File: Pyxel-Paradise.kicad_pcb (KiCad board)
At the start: 2 copper layers, 61 x 63.5 mm, 33 parts, among them J1 Joystick-North, J10 Action-Up, J11 Action-Right, J12 Action-Down, J13 Action-Left, J14 Meta-Button-1, J15 Meta-Button-2, J16 Meta-Button-3, J17 Meta-Button-4, J2 Joystick-NorthEast, J3 Joystick-East, J4 Joystick-SouthEast, J5 Joystick-South, J6 Joystick-SouthWest, J7 Joystick-West, J8 Joystick-NorthWest, J9 Raspberry_Pi_2_3

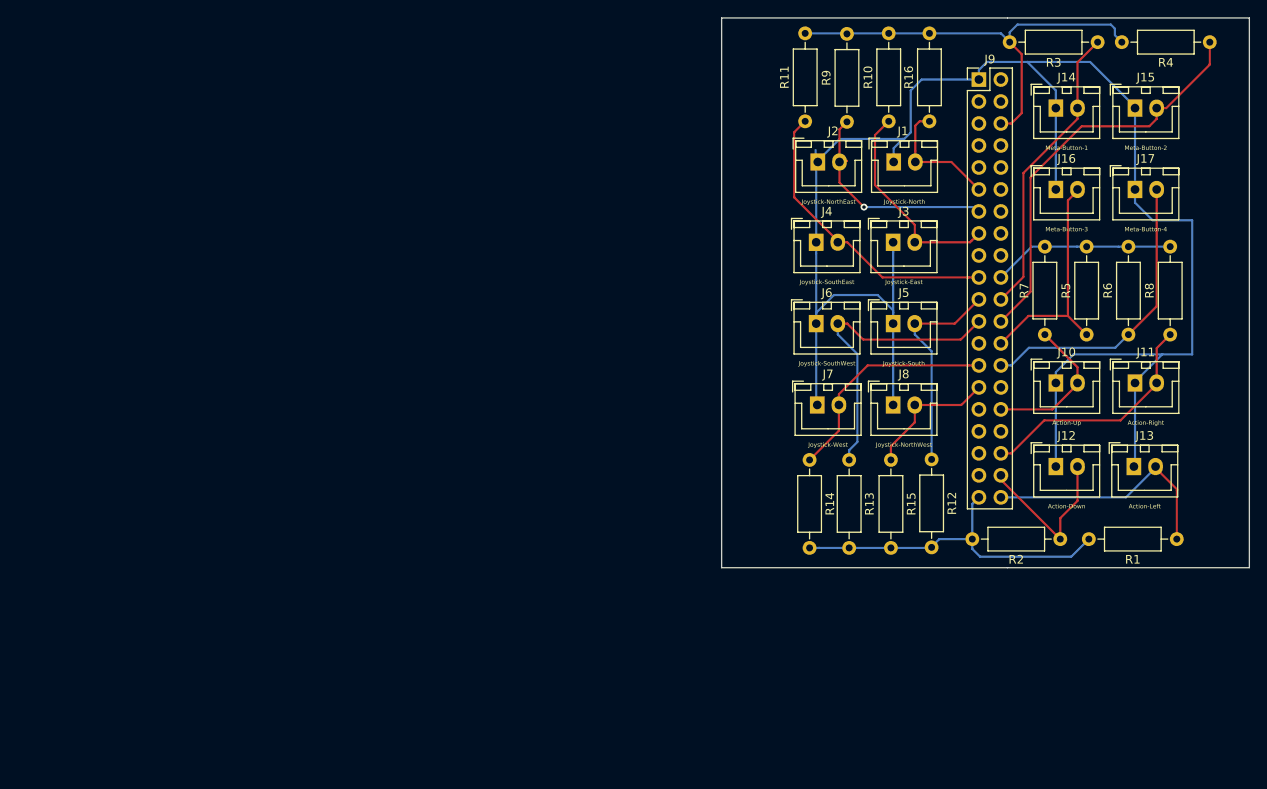
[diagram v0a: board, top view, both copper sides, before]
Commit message: V1 of a working PCB is complete
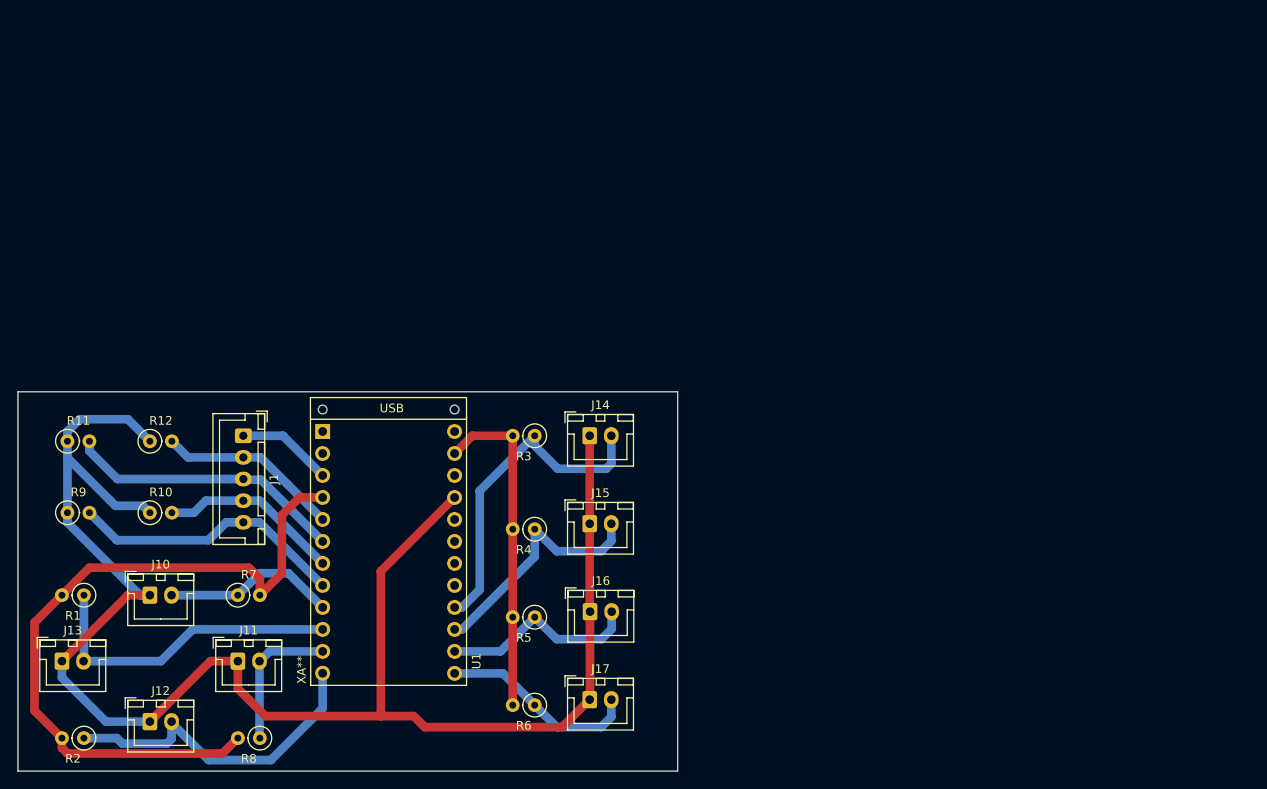
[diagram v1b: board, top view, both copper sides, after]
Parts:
- removed J2: Joystick-NorthEast, Connector_JST:JST_XH_B02B-XH-A_1x02_P2.50mm_Vertical
- removed J3: Joystick-East, Connector_JST:JST_XH_B02B-XH-A_1x02_P2.50mm_Vertical
- removed J4: Joystick-SouthEast, Connector_JST:JST_XH_B02B-XH-A_1x02_P2.50mm_Vertical
- removed J5: Joystick-South, Connector_JST:JST_XH_B02B-XH-A_1x02_P2.50mm_Vertical
- removed J6: Joystick-SouthWest, Connector_JST:JST_XH_B02B-XH-A_1x02_P2.50mm_Vertical
- removed J7: Joystick-West, Connector_JST:JST_XH_B02B-XH-A_1x02_P2.50mm_Vertical
- removed J8: Joystick-NorthWest, Connector_JST:JST_XH_B02B-XH-A_1x02_P2.50mm_Vertical
- removed J9: Raspberry_Pi_2_3, Connector_PinHeader_2.54mm:PinHeader_2x20_P2.54mm_Vertical
- removed R13, R14, R15, R16: 10k, Resistor_THT:R_Axial_DIN0207_L6.3mm_D2.5mm_P10.16mm_Horizontal
- added U1: Arduino_ProMicro_Socket, Arduino:Aruduino_ProMicro_Socket, F.Cu at (94.0, 119.4)
- J1: value Joystick-North -> Conn_01x05; footprint Connector_JST:JST_XH_B02B-XH-A_1x02_P2.50mm_Vertical -> Connector_JST:JST_XH_B05B-XH-A_1x05_P2.50mm_Vertical
- R1, R10, R11, R12, R2, R3, R4, R5, R6, R7, R8, R9: footprint Resistor_THT:R_Axial_DIN0207_L6.3mm_D2.5mm_P10.16mm_Horizontal -> Resistor_THT:R_Axial_DIN0207_L6.3mm_D2.5mm_P2.54mm_Vertical
- moved R1 126.4 mm to (58.4, 125.1)
- moved J13 125.8 mm to (55.9, 132.7)
- moved R2 115.1 mm to (58.4, 141.6)
- moved R8 115.0 mm to (78.7, 141.6), turned to 180 degrees
- moved J12 108.7 mm to (66.0, 139.7)
- moved J11 108.5 mm to (76.2, 132.7)
- moved J10 107.5 mm to (66.0, 125.1)
- moved R9 100.7 mm to (56.5, 115.6), turned to 0 degrees
- moved R7 98.0 mm to (76.2, 125.1), turned to 0 degrees
- moved R10 96.6 mm to (66.0, 115.6), turned to 0 degrees
- moved R4 96.2 mm to (110.5, 117.5)
- moved R11 92.9 mm to (56.5, 107.3), turned to 0 degrees
- moved R12 90.3 mm to (66.0, 107.3), turned to 0 degrees
- moved J17 86.3 mm to (116.8, 137.2)
- moved J1 81.5 mm to (76.8, 106.7), turned to 270 degrees
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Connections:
- J1 pad 1: +3V3 -> GND
- J1 pad 2: /North -> /JOYSTICK_NORTH
- J10 pad 1: +3V3 -> VCC
- J11 pad 1: +3V3 -> VCC
- J12 pad 1: +3V3 -> VCC
- J13 pad 1: +3V3 -> VCC
- J14 pad 1: +3V3 -> VCC
- J15 pad 1: +3V3 -> VCC
- J16 pad 1: +3V3 -> VCC
- J17 pad 1: +3V3 -> VCC
- R10 pad 1: /East -> VCC
- R10 pad 2: GND -> /JOYSTICK_WEST
- R11 pad 1: /SouthEast -> VCC
- R11 pad 2: GND -> /JOYSTICK_SOUTH
- R12 pad 1: /South -> VCC
- R12 pad 2: GND -> /JOYSTICK_NORTH
- R9 pad 1: /NorthEast -> VCC
- R9 pad 2: GND -> /JOYSTICK_EAST
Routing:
- net +3V3: track 205.1 -> 0.00 mm
- net VCC: track 0.00 -> 193.6 mm
- net /SouthWest: track 35.0 -> 0.00 mm
- net /SouthEast: track 34.6 -> 0.00 mm
- net /JOYSTICK_SOUTH: track 0.00 -> 32.4 mm
- net /JOYSTICK_EAST: track 0.00 -> 32.1 mm
- net /West: track 26.5 -> 0.00 mm
- net /NorthEast: track 26.0 -> 0.00 mm, vias 1 -> 0
- net /South: track 25.1 -> 0.00 mm
- net /East: track 24.4 -> 0.00 mm
- net /JOYSTICK_NORTH: track 0.00 -> 21.2 mm
- net GND: track 112.7 -> 133.8 mm
- net /JOYSTICK_WEST: track 0.00 -> 21.0 mm
- net /Meta-Button-2: track 47.5 -> 28.3 mm
- net /Action-Button-Down: track 19.4 -> 38.5 mm
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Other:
- board size 61 x 63.5 mm -> 76.2 x 43.8 mm
